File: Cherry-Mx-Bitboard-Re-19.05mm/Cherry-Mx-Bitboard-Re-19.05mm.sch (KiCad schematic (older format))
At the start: 22 parts, among them SW1 SW_Push, SW2 SW_Push-Switch

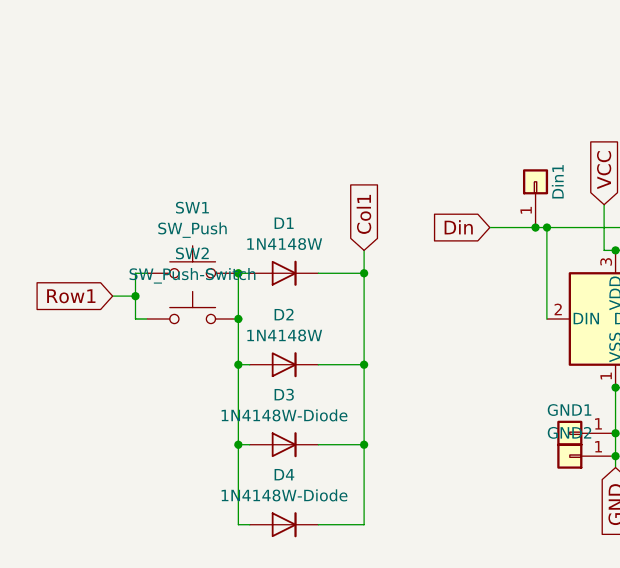
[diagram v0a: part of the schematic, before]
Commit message: simplified
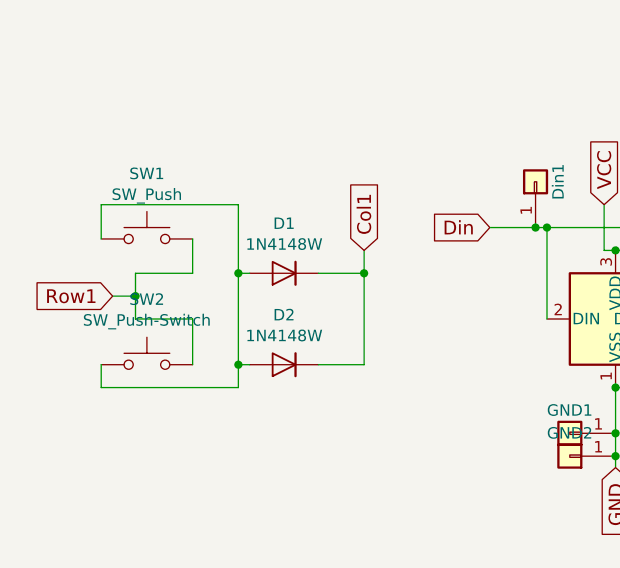
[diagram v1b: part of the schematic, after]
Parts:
- removed D3, D4: 1N4148W-Diode, Footprints:1N4148W, symbol Cherry-Mx-Bitboard-Re-19.05mm-rescue:1N4148W-Diode
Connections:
- net Row1: now also SW1.2, SW2.2; no longer SW1.1, SW2.1
- net at D1.2 (A), D2.2 (A): now also SW1.1, SW2.1; no longer SW1.2, SW2.2
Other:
- moved on the sheet: SW1, SW2
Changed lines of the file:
@@
 L Cherry-Mx-Bitboard-Re-19.05mm-rescue:SW_Push-Switch SW1
 U 1 1 5B598EC8
-P 2000 4500
-F 0 "SW1" H 2000 4785 50  0000 C CNN
-F 1 "SW_Push" H 2000 4694 50  0000 C CNN
-F 2 "Footprints:CherryMx_Socket" H 2000 4700 50  0001 C CNN
-F 3 "" H 2000 4700 50  0001 C CNN
-	1    2000 4500
+P 1800 4350
+F 0 "SW1" H 1800 4635 50  0000 C CNN
+F 1 "SW_Push" H 1800 4544 50  0000 C CNN
+F 2 "Footprints:CherryMx_Socket" H 1800 4550 50  0001 C CNN
+F 3 "" H 1800 4550 50  0001 C CNN
+	1    1800 4350
 	1    0    0    -1
 $EndComp
 Wire Wire Line
 	2200 4500 2250 4500
-Wire Wire Line
-	1800 4500 1750 4500
 Wire Wire Line
 	1750 4500 1750 4600
@@
 	2550 4900 2750 4900
 Wire Wire Line
-	2200 4900 2200 4700
-Connection ~ 2200 4500
-Wire Wire Line
 	2750 4900 2750 4500
 Connection ~ 2750 4500
@@
 L Cherry-Mx-Bitboard-Re-19.05mm-rescue:SW_Push-Switch SW2
 U 1 1 5EAC5567
-P 2000 4700
-F 0 "SW2" H 2000 4985 50  0000 C CNN
-F 1 "SW_Push-Switch" H 2000 4894 50  0000 C CNN
-F 2 "keyswitches:Kailh_socket_PG1350" H 2000 4900 50  0001 C CNN
-F 3 "" H 2000 4900 50  0001 C CNN
-	1    2000 4700
-	1    0    0    -1
-$EndComp
-Connection ~ 2200 4700
-Wire Wire Line
-	2200 4700 2200 4500
-Wire Wire Line
-	1800 4700 1750 4700
+P 1800 4900
+F 0 "SW2" H 1800 5185 50  0000 C CNN
+F 1 "SW_Push-Switch" H 1800 5094 50  0000 C CNN
+F 2 "keyswitches:Kailh_socket_PG1350" H 1800 5100 50  0001 C CNN
+F 3 "" H 1800 5100 50  0001 C CNN
+	1    1800 4900
+	1    0    0    -1
+$EndComp
 Wire Wire Line
 	1750 4700 1750 4600
 Connection ~ 1750 4600
-$Comp
-L Cherry-Mx-Bitboard-Re-19.05mm-rescue:1N4148W-Diode D3
-U 1 1 5EAE37ED
-P 2400 5250
-F 0 "D3" H 2400 5467 50  0000 C CNN
-F 1 "1N4148W-Diode" H 2400 5376 50  0000 C CNN
-F 2 "Footprints:1N4148W" H 2400 5075 50  0001 C CNN
-F 3 "" H 2400 5250 50  0001 C CNN
-	1    2400 5250
-	-1   0    0    -1
-$EndComp
-Wire Wire Line
-	2550 5250 2750 5250
-Wire Wire Line
-	2750 5250 2750 4900
-Connection ~ 2750 4900
-Wire Wire Line
-	2250 5250 2200 5250
-Wire Wire Line
-	2200 5250 2200 4900
-Connection ~ 2200 4900
-$Comp
-L Cherry-Mx-Bitboard-Re-19.05mm-rescue:1N4148W-Diode D4
-U 1 1 5EAE84E4
-P 2400 5600
-F 0 "D4" H 2400 5817 50  0000 C CNN
-F 1 "1N4148W-Diode" H 2400 5726 50  0000 C CNN
-F 2 "Footprints:1N4148W" H 2400 5425 50  0001 C CNN
-F 3 "" H 2400 5600 50  0001 C CNN
-	1    2400 5600
-	-1   0    0    -1
-$EndComp
-Wire Wire Line
-	2550 5600 2750 5600
-Wire Wire Line
-	2750 5600 2750 5250
-Connection ~ 2750 5250
-Wire Wire Line
-	2250 5600 2200 5600
-Wire Wire Line
-	2200 5600 2200 5250
-Connection ~ 2200 5250
 $Comp
 L LED:SK6812 D5
@@
 Wire Wire Line
 	3850 5300 3850 5200
+Wire Wire Line
+	2200 4500 2200 4900
+Wire Wire Line
+	2200 4500 2200 4200
+Wire Wire Line
+	2200 4200 1600 4200
+Wire Wire Line
+	1600 4200 1600 4350
+Connection ~ 2200 4500
+Wire Wire Line
+	2000 4350 2000 4500
+Wire Wire Line
+	1750 4500 2000 4500
+Wire Wire Line
+	2000 4700 2000 4900
+Wire Wire Line
+	1750 4700 2000 4700
+Wire Wire Line
+	1600 4900 1600 5000
+Wire Wire Line
+	1600 5000 2200 5000
+Wire Wire Line
+	2200 5000 2200 4900
+Connection ~ 2200 4900
 $EndSCHEMATC
